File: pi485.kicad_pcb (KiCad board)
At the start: 2 copper layers, 53 x 70 mm, 29 parts, among them J1 RS485, P1 Rasperry Pi, P2 PWR, P3 Term, Q1 2N4401, Q2 2N4401, Q3 2N4401, U1 NE555, U2 MAX485

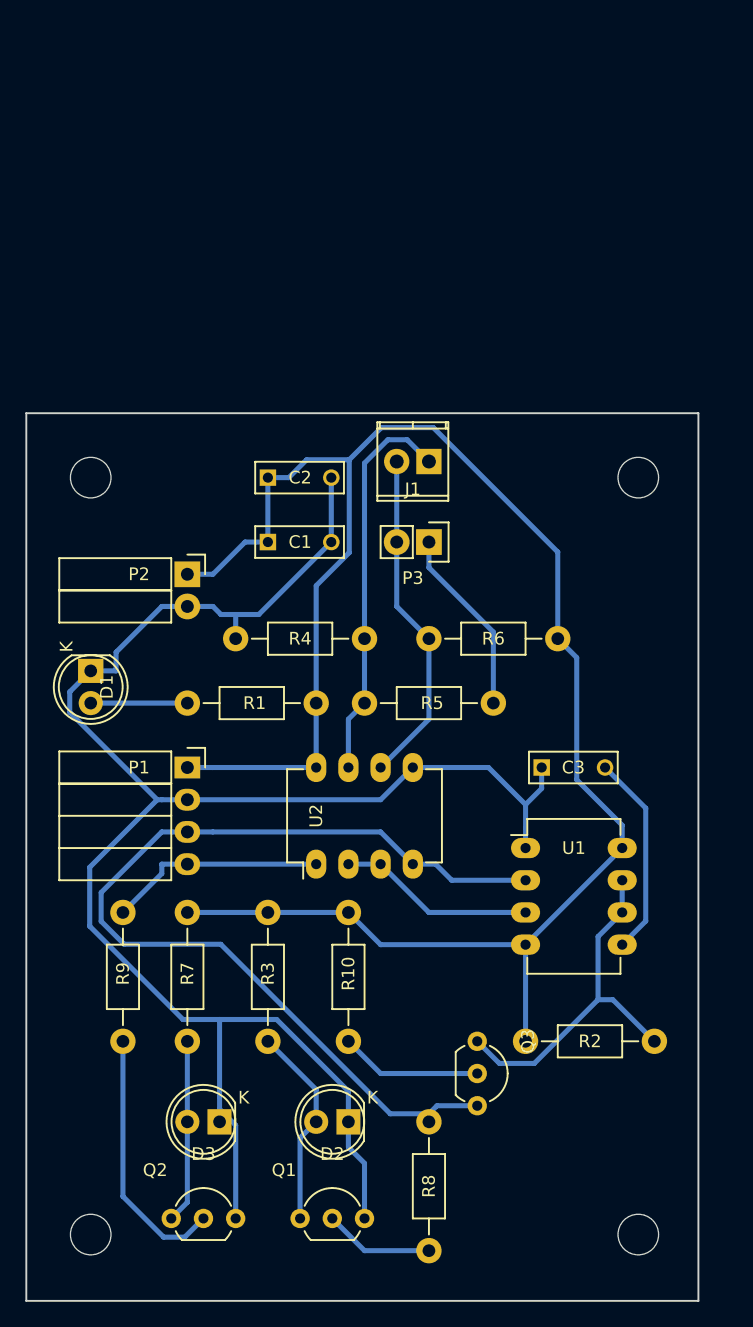
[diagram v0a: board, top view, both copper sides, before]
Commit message: Updating...
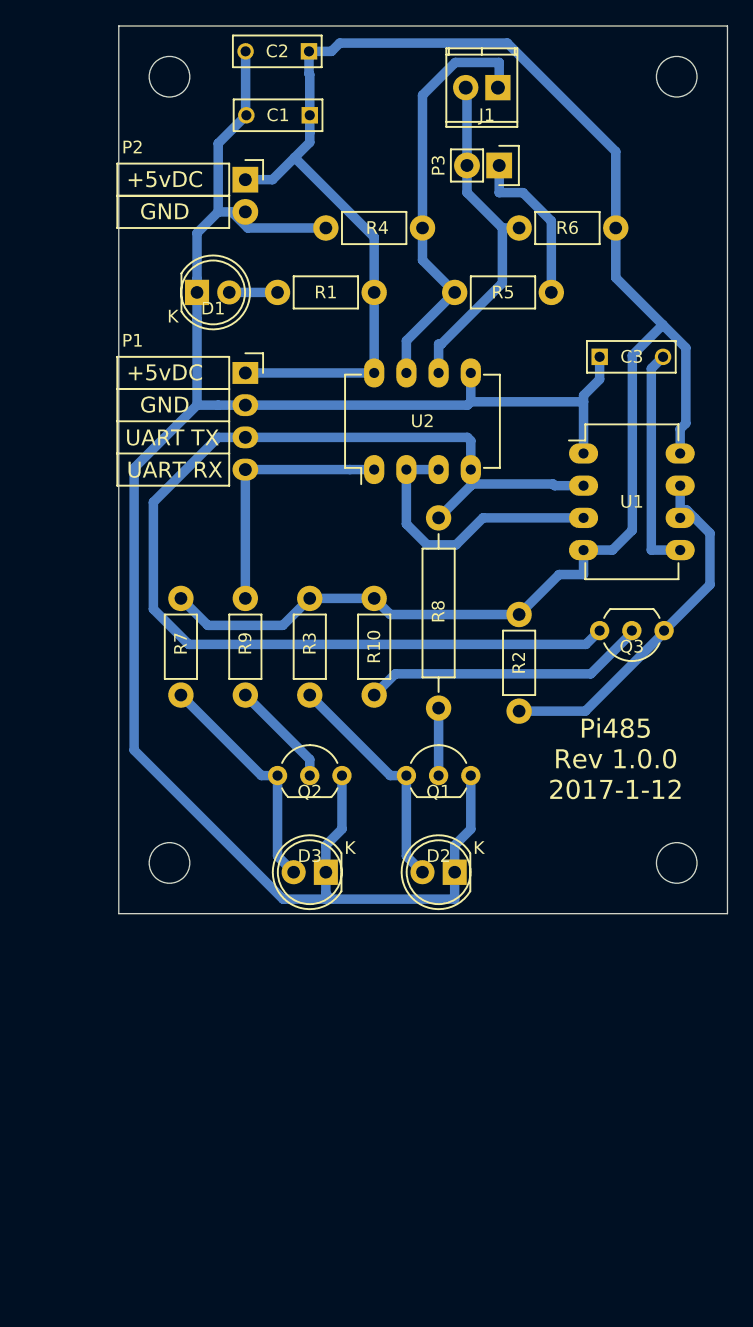
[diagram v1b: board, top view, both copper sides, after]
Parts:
- D1: value PWR -> PWRLED
- D2: value TX -> TXLED
- D3: value RX -> RXLED
- Q1, Q2, Q3: value 2N4401 -> 2N2222
- R1, R10, R2, R3, R4, R5, R6, R7, R9: footprint Resistors_THT:Resistor_Horizontal_RM10mm -> Resistors_THT:Resistor_Horizontal_RM7mm
- R8: footprint Resistors_THT:Resistor_Horizontal_RM10mm -> Resistors_THT:Resistor_Horizontal_RM15mm
- moved R8 42.8 mm to (109.2, 112.8)
- moved Q1 35.9 mm to (106.7, 118.1)
- moved Q2 35.9 mm to (96.5, 118.1)
- moved Q3 35.6 mm to (127.0, 106.7), turned to 180 degrees
- moved C1 33.8 mm to (99.1, 66.0), turned to 180 degrees
- moved C2 33.8 mm to (99.0, 61.0), turned to 180 degrees
- moved R4 33.2 mm to (100.3, 74.9)
- moved R5 33.2 mm to (110.5, 80.0)
- moved R6 33.2 mm to (115.6, 74.9)
- moved C3 32.7 mm to (121.9, 85.1)
- moved R1 32.7 mm to (104.1, 80.0)
- moved REF01 32.2 mm to (88.0, 63.0)
- moved REF02 31.8 mm to (128.0, 63.0)
- moved U1 31.4 mm to (120.7, 92.7)
- moved P1 31.4 mm to (94.0, 86.4)
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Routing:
- net /(TXDO)_GPIO14: track 76.1 -> 88.6 mm
- net Net-(Q2-Pad2): track 20.5 -> 8.45 mm
- net GND: track 149.2 -> 160.8 mm
- net Net-(Q3-Pad2): track 11.2 -> 22.5 mm
- net VCC: track 148.1 -> 156.5 mm
- net Net-(U1-Pad3): track 15.5 -> 22.4 mm
- net Net-(D3-Pad2): track 14.5 -> 18.4 mm
- net Net-(D1-Pad2): track 7.62 -> 3.81 mm
- net Net-(Q1-Pad2): track 8.67 -> 5.32 mm
- net /(RXDO)_GPIO15: track 17.3 -> 20.3 mm
- net Net-(J1-Pad1): track 31.1 -> 33.8 mm
- net Net-(D2-Pad2): track 16.1 -> 18.4 mm
- net Net-(P3-Pad1): track 14.8 -> 12.8 mm
- net Net-(C3-Pad2): track 16.1 -> 17.9 mm
- net Net-(Q3-Pad1): track 28.3 -> 29.5 mm
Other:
- board size 53 x 70 mm -> 48 x 70 mm
- net class Default: clearance 0.5 -> 0.75; trace_width 0.4 -> 0.75; via_dia 0.8 -> 1.2; via_drill 0.4 -> 0.8
- rule pad_to_mask_clearance: 1 -> 0
- rule trace_clearance: 0.5 -> 0.75
- rule trace_min: 0.4 -> 0.75
- rule via_min_drill: 0.3 -> 0.8
- rule via_min_size: 0.8 -> 1.2
- board text added: "+5vDC"
- board text added: "GND"
- board text added: "Pi485 Rev 1.0.0 2017-1-12"
- board text added: "UART RX"
- board text added: "UART TX"
